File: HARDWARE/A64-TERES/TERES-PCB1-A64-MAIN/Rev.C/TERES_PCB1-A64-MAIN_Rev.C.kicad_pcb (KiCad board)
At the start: 6 copper layers, 117 x 89 mm, 453 parts, among them CON1 CONN_01X40, CON2 CONN_01X06, CON3 CONN_01X20, CON4 CONN_01X40, Q1 12MHz-20pf, Q2 MC-306_32.768KHZ/SMD_8038/6pF, Q3 4SB24.000F20E15/5x3.2mm/20ppm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, Q4 27.000MHz/20ppm, T1 WPM1481(DFN2X2-6L), T2 DTC114YKA(SOT-23), U1 AllWinner-A64(FBGA396), U10 RCLAMP0524P(SLP2510P8), U11 RTL8723BS(ComboModule), U12 GL850G-SO28, U13 MT3608(SOT23-6), U14 AXP803(QFN68_8x8mm), U15 RCLAMP0524P(SLP2510P8), U16 MT3608(SOT23-6), U17 ANX6345, U18 TS4871, U19 TS4871, U2 K4B4G1646Q-HYK0(FBGA-96_256Mx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, U20 W25Q128FVSSIG, U21 SY6280AAC(SOT23-5), U3 K4B4G1646Q-HYK0(FBGA-96_256Mx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, U4 RCLAMP0524P(SLP2510P8), U5 MTFC4GACAANA-4M_IT(TBGA100), U6 TS5A23159, U7 RCLAMP0524P(SLP2510P8), U8 RCLAMP0524P(SLP2510P8), U9 SY6280AAC(SOT23-5)

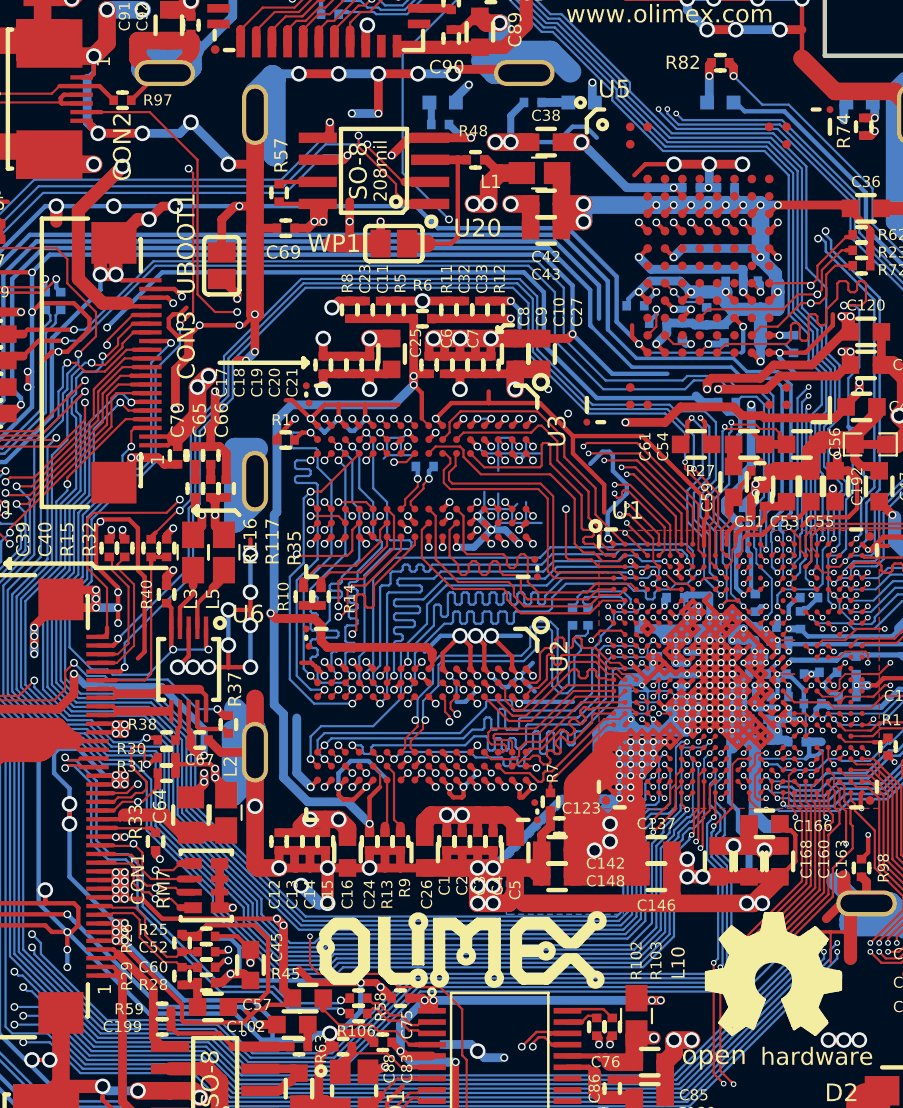
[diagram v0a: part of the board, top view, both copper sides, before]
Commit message: Update projects using KiCAD 6.0.7
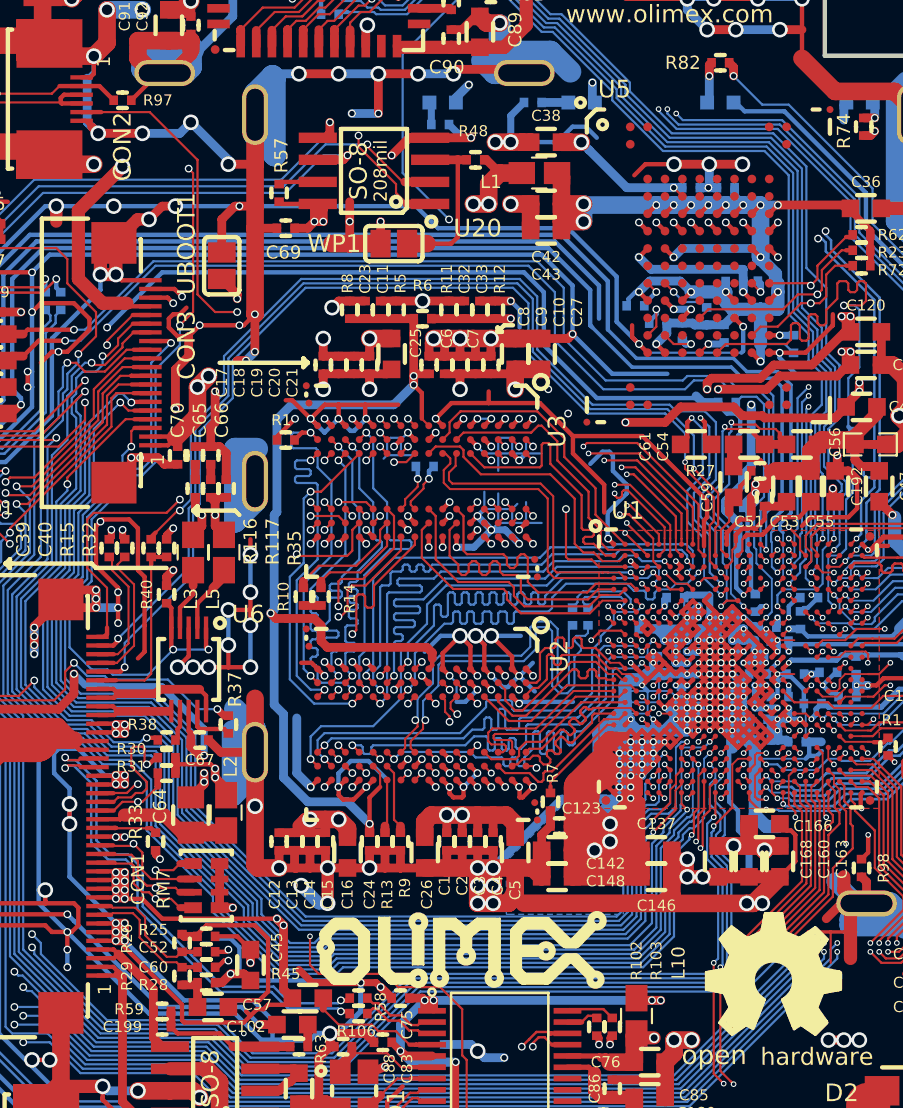
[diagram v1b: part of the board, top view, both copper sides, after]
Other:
- net class Default removed
